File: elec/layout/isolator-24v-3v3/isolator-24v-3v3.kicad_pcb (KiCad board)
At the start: 2 copper layers, 11 parts, among them U12 2.2µF ±10% 25V X7R, U2 8.2kΩ ±1% 62.5mW, U3 10kΩ ±1% 62.5mW, U5 10µH ±20%, U6 10µF ±10% 25V X5R, U7 10µF ±10% 25V X5R, U9 2.2µF ±10% 25V X7R

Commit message: restore layout files
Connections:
- net SW renamed cathode
- U12 pad 2: gnd-2 -> gnd-1
- U3 pad 1: hv-1 -> hv-2
- U4 pad 2: gnd-2 -> gnd-1
- U5 pad 2: hv-1 -> hv-2
- U6 pad 2: gnd-2 -> gnd-1
- U7 pad 1: hv-1 -> hv-2
- U8 pad 1: hv-2 -> hv-1
- U8 pad 2: gnd-1 -> gnd-2
- U8 pad 4: gnd-2 -> gnd-1
- U9 pad 1: hv-2 -> hv-1
- U9 pad 2: gnd-1 -> gnd-2
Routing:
- net gnd-2: track 26.0 -> 3.04 mm, vias 3 -> 0
- net gnd-1: track 3.04 -> 26.0 mm, vias 0 -> 3
- net hv-2: track 2.88 -> 0.00 mm
- net hv-1: track 0.00 -> 2.88 mm

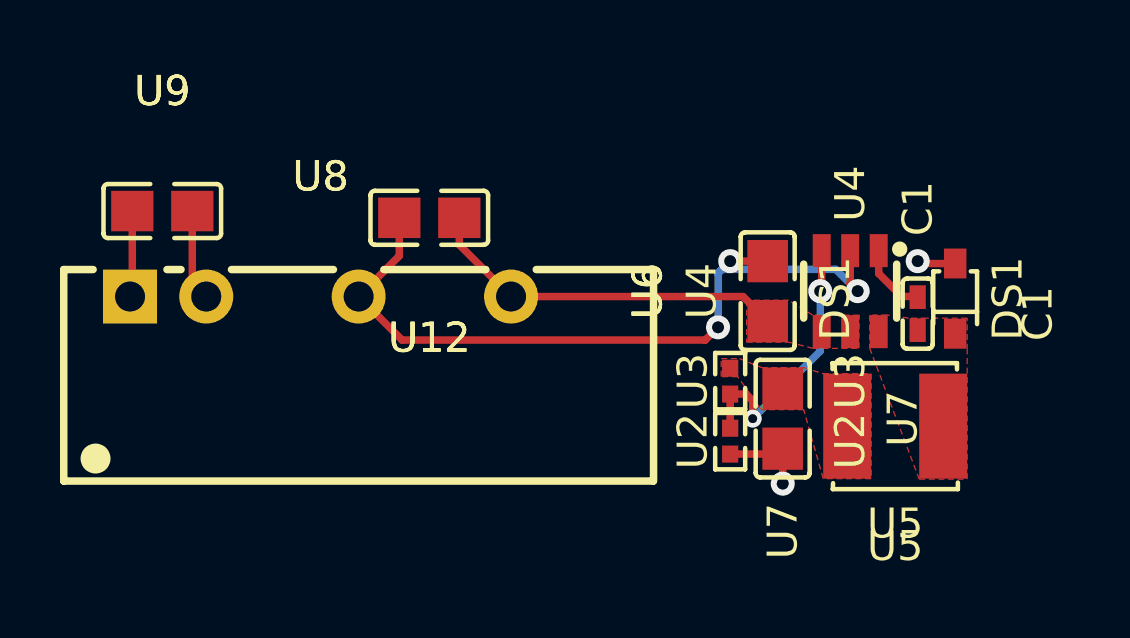
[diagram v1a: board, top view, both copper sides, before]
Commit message: building frozen
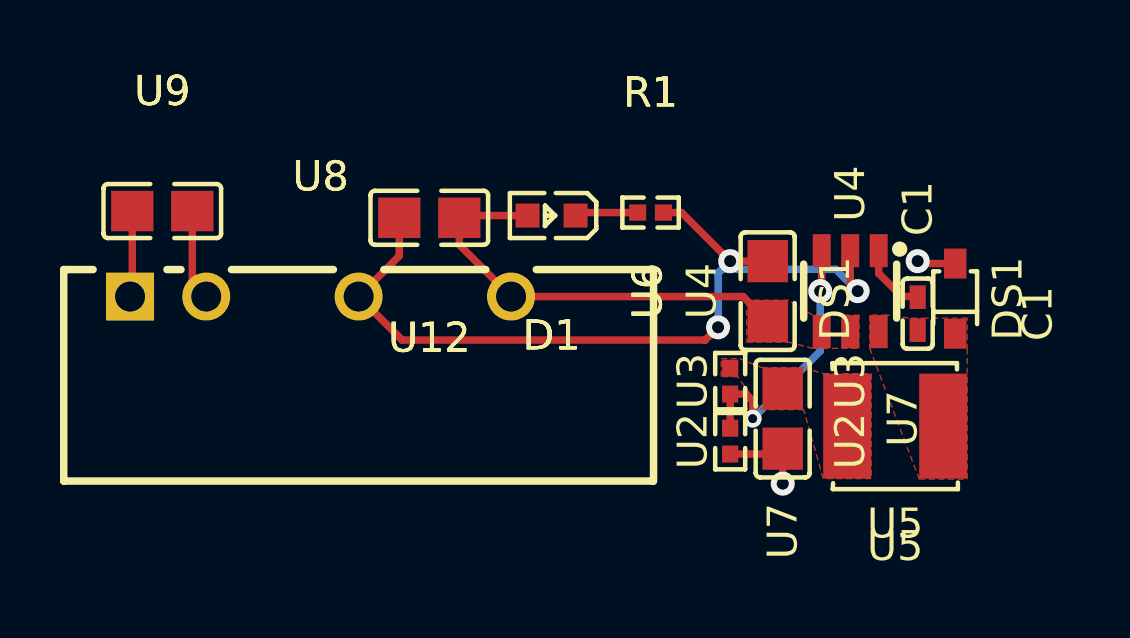
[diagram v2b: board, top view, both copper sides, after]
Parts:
- added D1: , atopile:LED0603-RD-c81ffb, F.Cu at (94.2, 87.3)
- added R1: 1kΩ ±1% 62.5mW, atopile:R0402-56259e, F.Cu at (97.5, 87.2)
- U12: value 2.2µF ±10% 25V X7R -> 10µF ±10% 25V X5R
- U2: value 8.2kΩ ±1% 62.5mW -> 10kΩ ±1% 62.5mW
- U6: value 10µF ±10% 25V X5R -> 4.7µF ±10% 25V X5R
- U8: footprint atopile:PWRM-TH_BXXXXS-2WR3-d8b2fb -> atopile:PWRM-TH_BXXXXS-2WR2-87119e
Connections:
- net cathode renamed SW
- net line renamed FB
- DS1 pad 2: gnd -> gnd-2
- U12 pad 2: gnd-1 -> gnd
- U2 pad 2: gnd -> gnd-2
- U3 pad 1: hv-2 -> hv-1
- U4 pad 2: gnd-1 -> gnd
- U5 pad 2: hv-2 -> hv-1
- U6 pad 2: gnd-1 -> gnd
- U7 pad 1: hv-2 -> hv-1
- U7 pad 2: gnd -> gnd-2
- U8 pad 1: hv-1 -> hv-2
- U8 pad 2: gnd-2 -> gnd-1
- U8 pad 4: gnd-1 -> gnd
- U9 pad 1: hv-1 -> hv-2
- U9 pad 2: gnd-2 -> gnd-1
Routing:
- net gnd: track 4.28 -> 28.9 mm, vias 2 -> 3
- net gnd-1: track 26.0 -> 3.04 mm, vias 3 -> 0
- net hv-2: track 0.00 -> 2.88 mm
- net hv-1: track 2.88 -> 0.00 mm
- net hv: track 12.2 -> 14.5 mm
- net cathode: track 0.00 -> 2.11 mm
- net gnd-2: track 3.04 -> 4.28 mm, vias 0 -> 2
